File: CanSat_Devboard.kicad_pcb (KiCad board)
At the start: 4 copper layers, 64.1 x 43.6 mm, 49 parts, among them IC1 114993390, J1 I2C, J3 Conn_01x03_Pin, J4 USB_C_Receptacle_USB2.0_16P, J5 693071010811, J6 SWD, J7 RMF, J8 GPIO, SW3 SW_Push, SW4 SHPHLD, SW5 RST, U1 E73-2G4M08S1C, U3 SRV05-4, U4 NPM1300-QEAA-R7, Y1 32.768

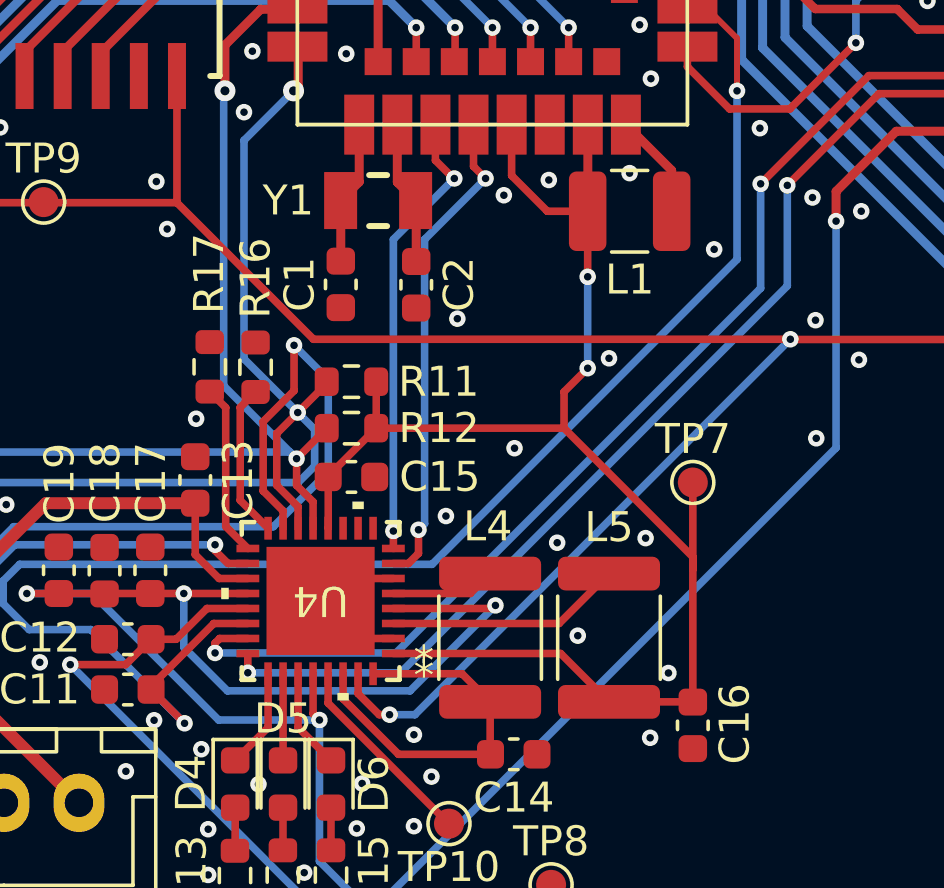
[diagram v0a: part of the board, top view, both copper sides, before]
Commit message: Fixed a roouting mistake
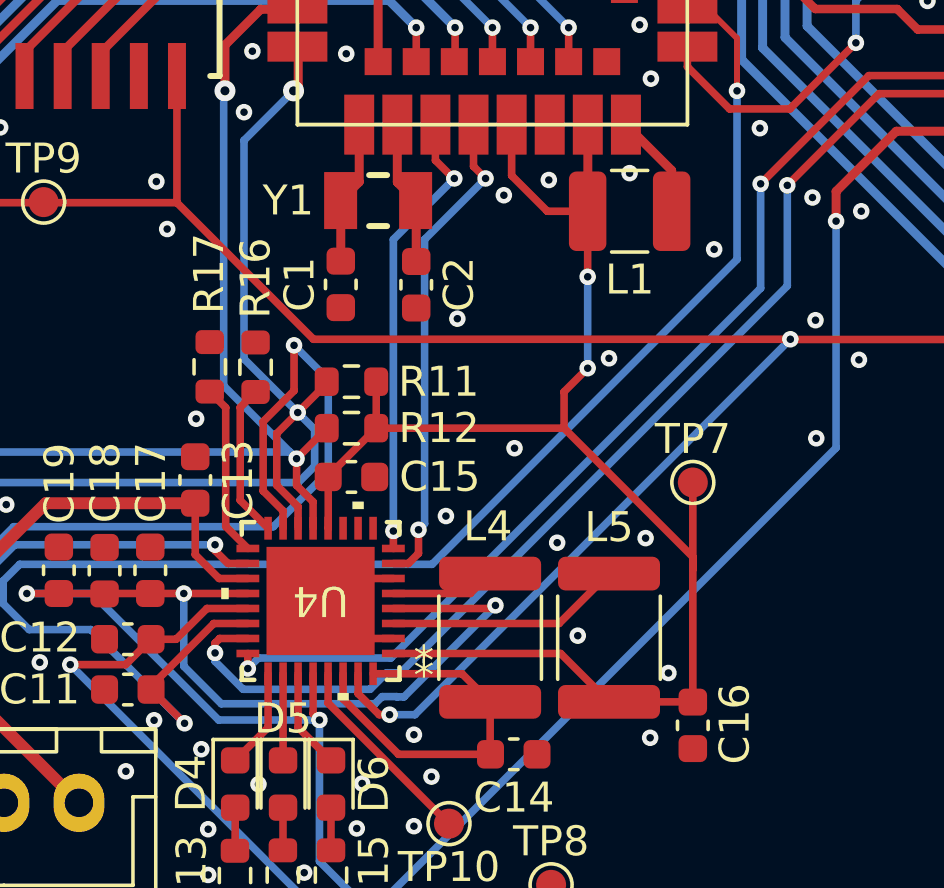
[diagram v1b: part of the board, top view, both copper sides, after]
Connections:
- J8 pad 14: 0.08 -> unconnected-(J8-Pin_14-Pad14)
- U4 pad 23: CC2 -> CC1
- U4 pad 24: CC1 -> CC2
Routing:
- net CC1: track 45.8 -> 48.7 mm
- net CC2: track 48.2 -> 46.4 mm
- net VSYS: track 55.1 -> 55.9 mm
